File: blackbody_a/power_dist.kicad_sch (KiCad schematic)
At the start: 21 parts, among them IC2 TPS562231DRLR, U4 RO-123.3S_HP

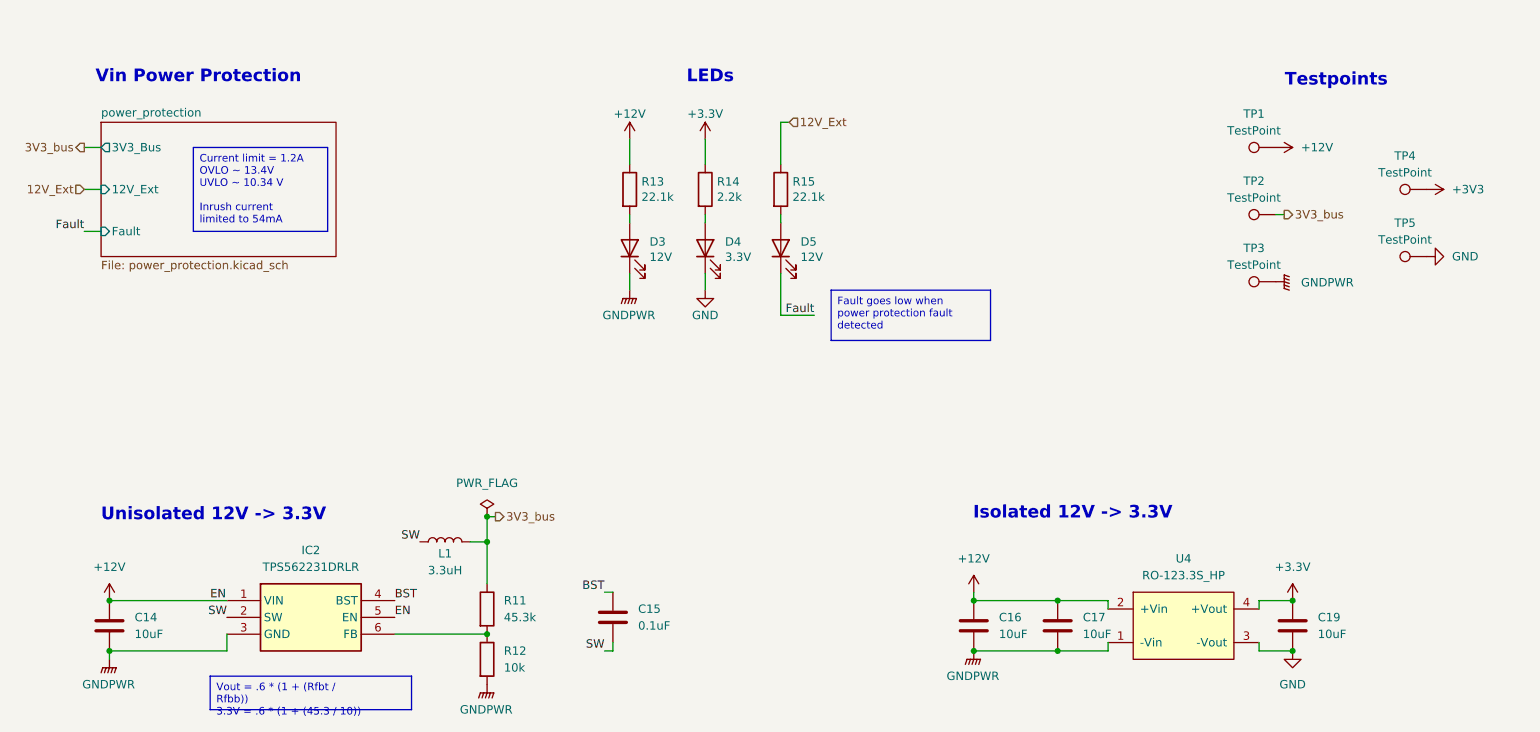
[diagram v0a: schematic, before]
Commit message: Fixed pins, minor changes, removed power isolation
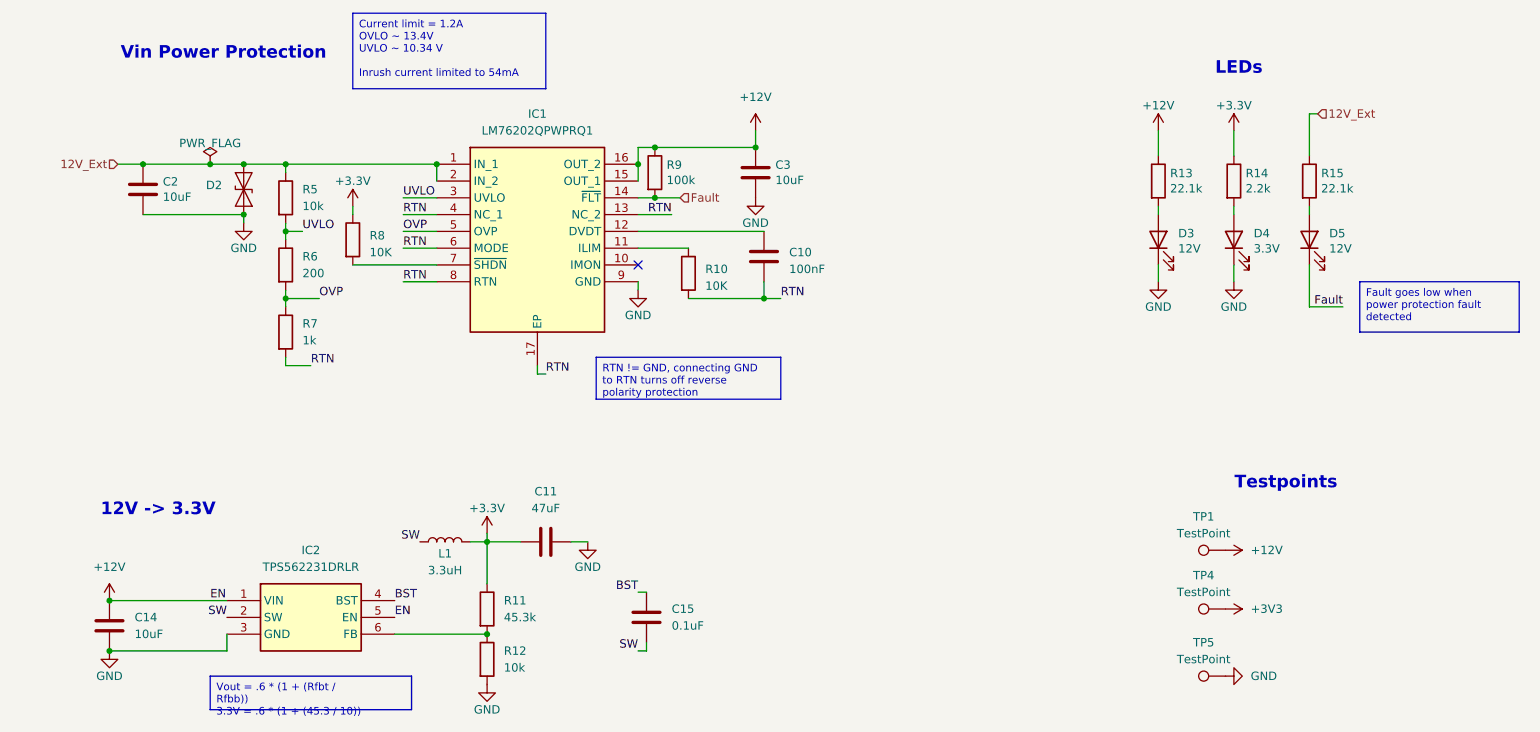
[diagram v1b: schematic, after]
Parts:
- removed C16, C17, C19: 10uF, symbol Device:C
- removed TP2, TP3: TestPoint, symbol Connector:TestPoint
- removed U4: RO-123.3S_HP, UTSVT_ICs:RI3_DC_Converter, symbol utsvt-power-regulators:RO-123.3S_HP
- added C10: 100nF, Capacitor_SMD:C_0805_2012Metric, symbol Device:C
- added C11: 47uF, symbol Device:C
- added C2, C3: 10uF, Capacitor_SMD:C_0805_2012Metric, symbol Device:C
- added D2: SD12_SOD323, Diode_SMD:D_SOD-323, symbol Diode:SD12_SOD323
- added IC1: LM76202QPWPRQ1, SOP65P640X120-17N, symbol LM76202QPWPRQ1:LM76202QPWPRQ1
- added R10, R8: 10K, Resistor_SMD:R_0805_2012Metric, symbol Device:R
- added R5: 10k, Resistor_SMD:R_0805_2012Metric, symbol Device:R
- added R6: 200, Resistor_SMD:R_0805_2012Metric, symbol Device:R
- added R7: 1k, Resistor_SMD:R_0805_2012Metric, symbol Device:R
- added R9: 100k, Resistor_SMD:R_0805_2012Metric, symbol Device:R
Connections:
- net 3V3_bus is gone; now on net +3.3V: L1.2, R11.1
- net GNDPWR is gone; now on net GND: C14.2, D3.1 (K), IC2.3 (GND), R12.2
- net +12V: now also C3.1, IC1.15 (OUT_1), IC1.16 (OUT_2), R9.1
- net +3.3V: now also C11.1, R8.1
- net 12V_Ext: now also C2.1, D2.2 (A2), IC1.1 (IN_1), IC1.2 (IN_2), R5.1
- net Fault: now also IC1.14 (~{FLT}), R9.2
- net GND: now also C11.2, C2.2, C3.2, D2.1 (A1), IC1.9 (GND)
- new net: IC1.11 (ILIM), R10.1
- new net: C10.1, IC1.12 (DVDT)
- new net: IC1.7 (~{SHDN}), R8.2
- new net OVP: IC1.5 (OVP), R6.2, R7.1
- new net RTN: C10.2, IC1.13 (NC_2), IC1.17 (EP), IC1.4 (NC_1), IC1.6 (MODE), IC1.8 (RTN), R10.2, R7.2
- new net UVLO: IC1.3 (UVLO), R5.2, R6.1
- no-connect marks 0 -> 1
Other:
- removed sheet power_protection
- note added: "12V -> 3.3V"
- note removed: "Isolated 12V -> 3.3V"
- note removed: "Unisolated 12V -> 3.3V"
- moved on the sheet: C15, D3, D4, D5, R13, R14, R15, TP1, TP4, TP5

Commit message: layout iteration 1
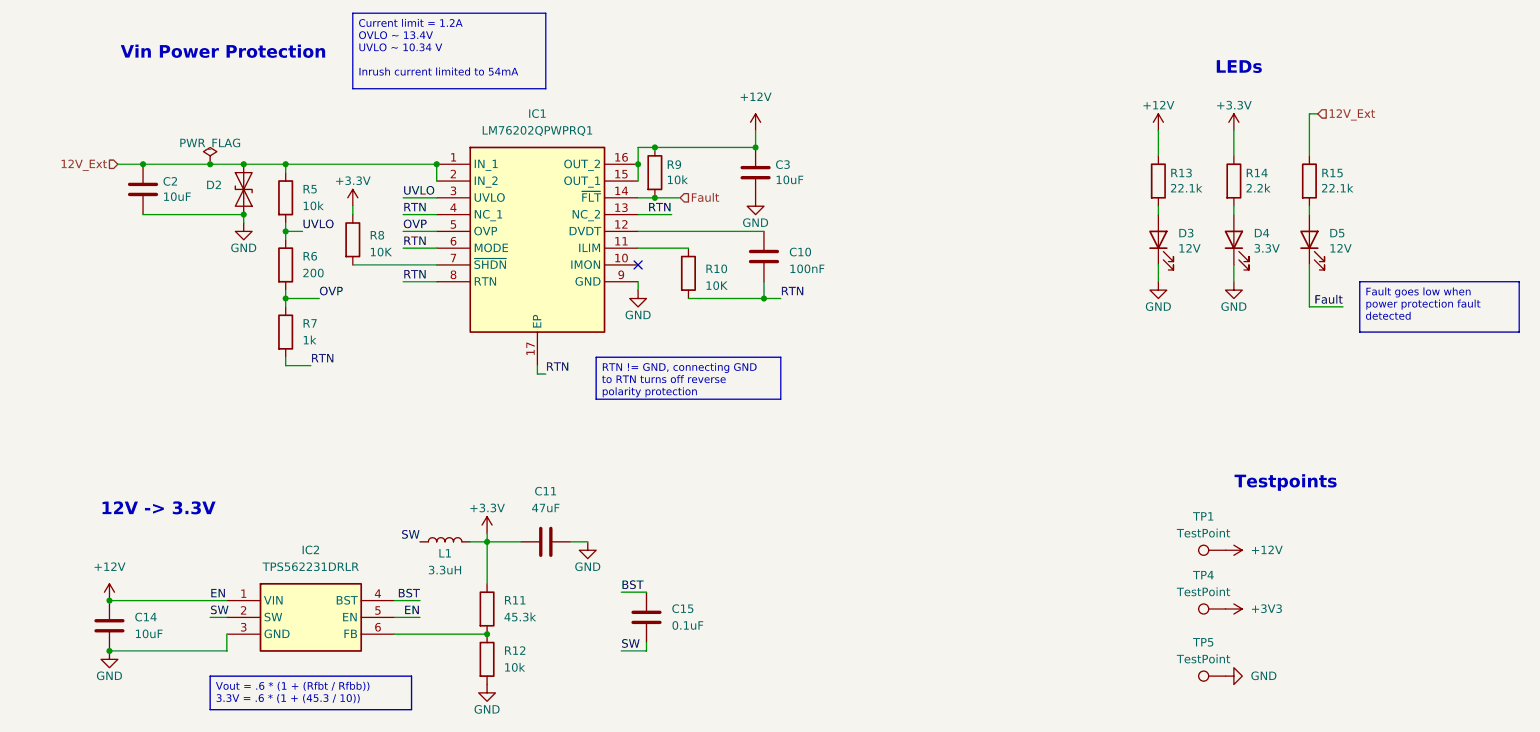
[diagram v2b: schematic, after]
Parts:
- C11, C14, C15: footprint (none) -> Capacitor_SMD:C_0805_2012Metric
- IC1: footprint SOP65P640X120-17N -> blackbody_a:LM76202QPWPRQ1
- IC2: footprint SOTFL50P160X60-6N -> blackbody_a:TPS562231DRLR
- L1: footprint (none) -> Inductor_SMD:L_0805_2012Metric
- R9: value 100k -> 10k
- TP1, TP4, TP5: footprint (none) -> TestPoint:TestPoint_Pad_D1.0mm
